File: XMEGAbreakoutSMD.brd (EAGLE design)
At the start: 160 x 100 mm, 23 parts, among them IC1 XMEGA16A4

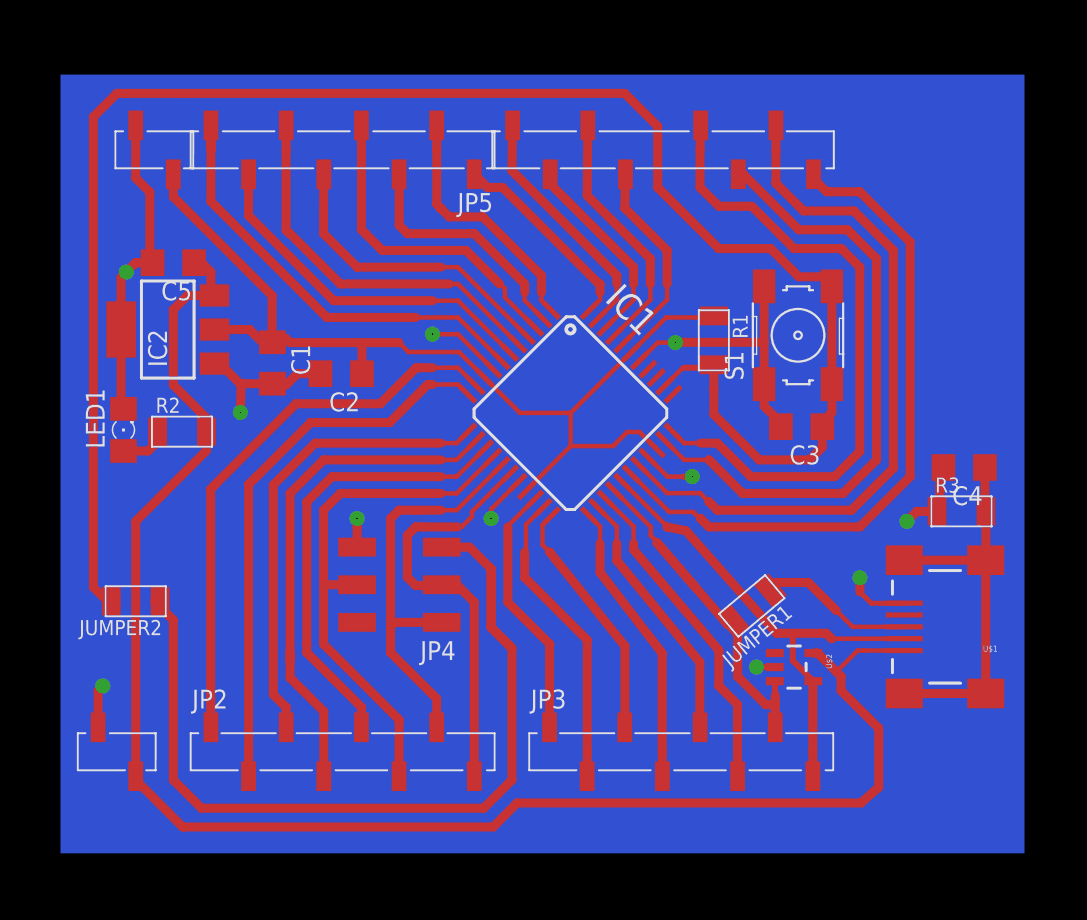
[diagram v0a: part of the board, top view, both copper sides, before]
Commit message: latest
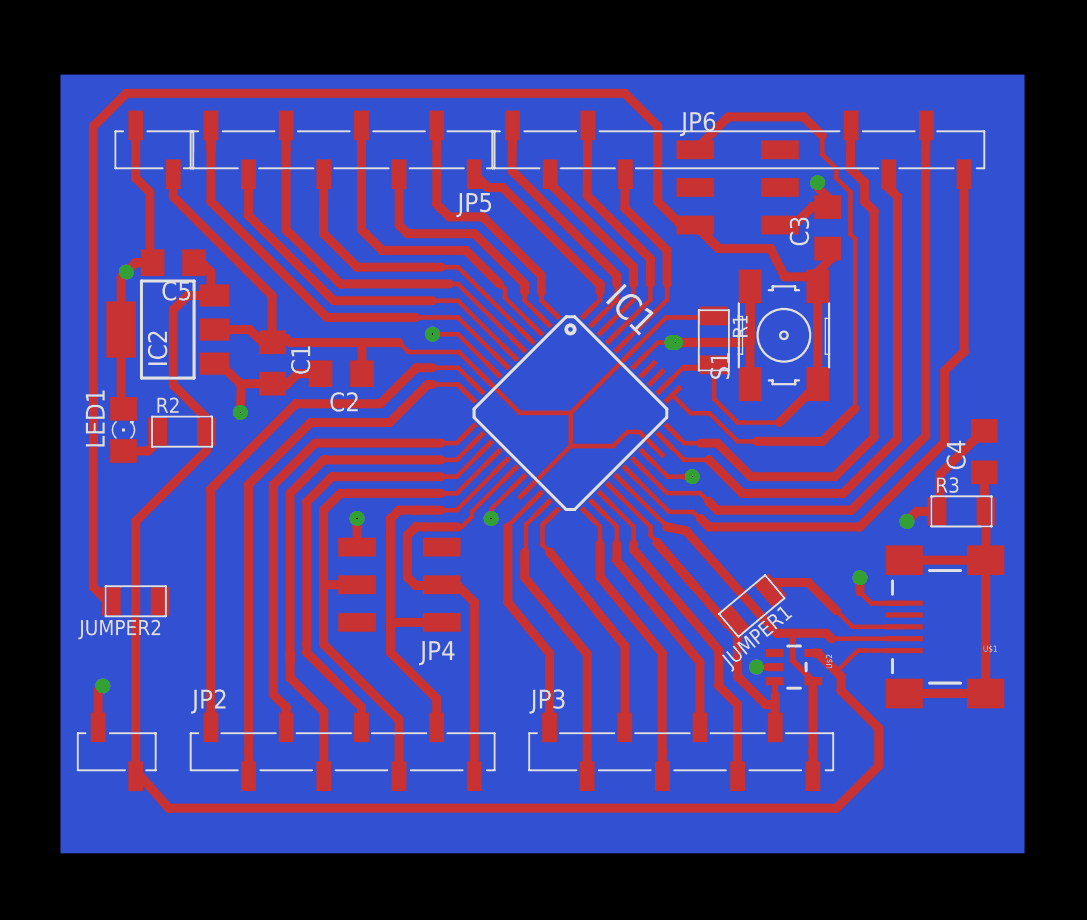
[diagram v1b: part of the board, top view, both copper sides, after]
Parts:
- added JP6: (no value), fab:2X03SMD
- moved C3 13.5 mm to (91.2, 57.0), turned to 90 degrees
- moved JP1 10.2 mm to (100.4, 62.2)
- moved C4 1.73 mm to (101.7, 41.9), turned to 90 degrees
- moved S1 0.95 mm to (88.2, 49.7)
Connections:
- new net DAT: IC1.34, JP6.1
- net GND: now also JP6.6
- net RESET: now also JP6.5; no longer JP4.5
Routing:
- net RESET: track 180.5 -> 117.7 mm
- net DAT: track 0.00 -> 43.9 mm
- net GND: track 218.0 -> 246.7 mm, vias 11 -> 12
- net PE3: track 44.2 -> 37.6 mm
- net PE2: track 42.2 -> 36.9 mm
- net PE1: track 48.0 -> 43.6 mm
- net PE0: track 45.9 -> 43.7 mm
- net VBUS: track 111.5 -> 109.3 mm
